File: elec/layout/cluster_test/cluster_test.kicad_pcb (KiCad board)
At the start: 2 copper layers, 31 parts

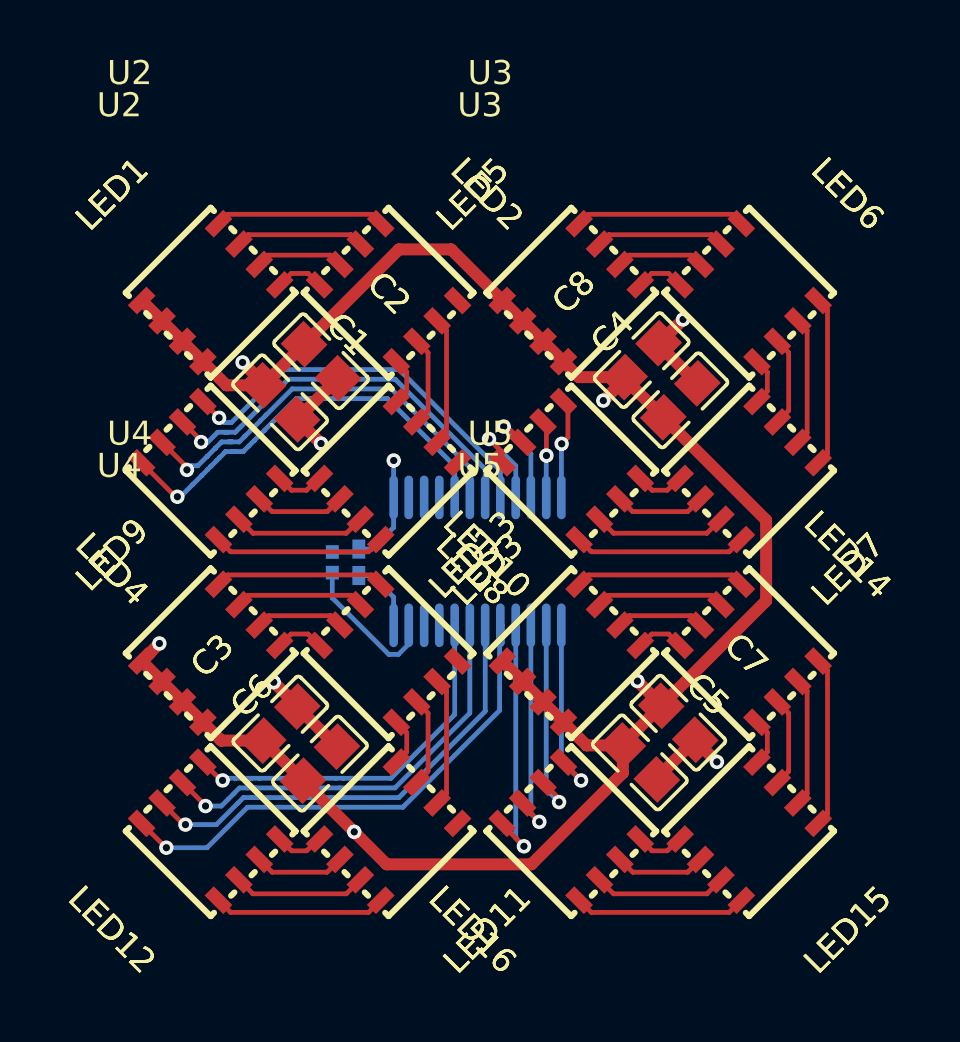
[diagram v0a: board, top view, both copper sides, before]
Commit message: built this
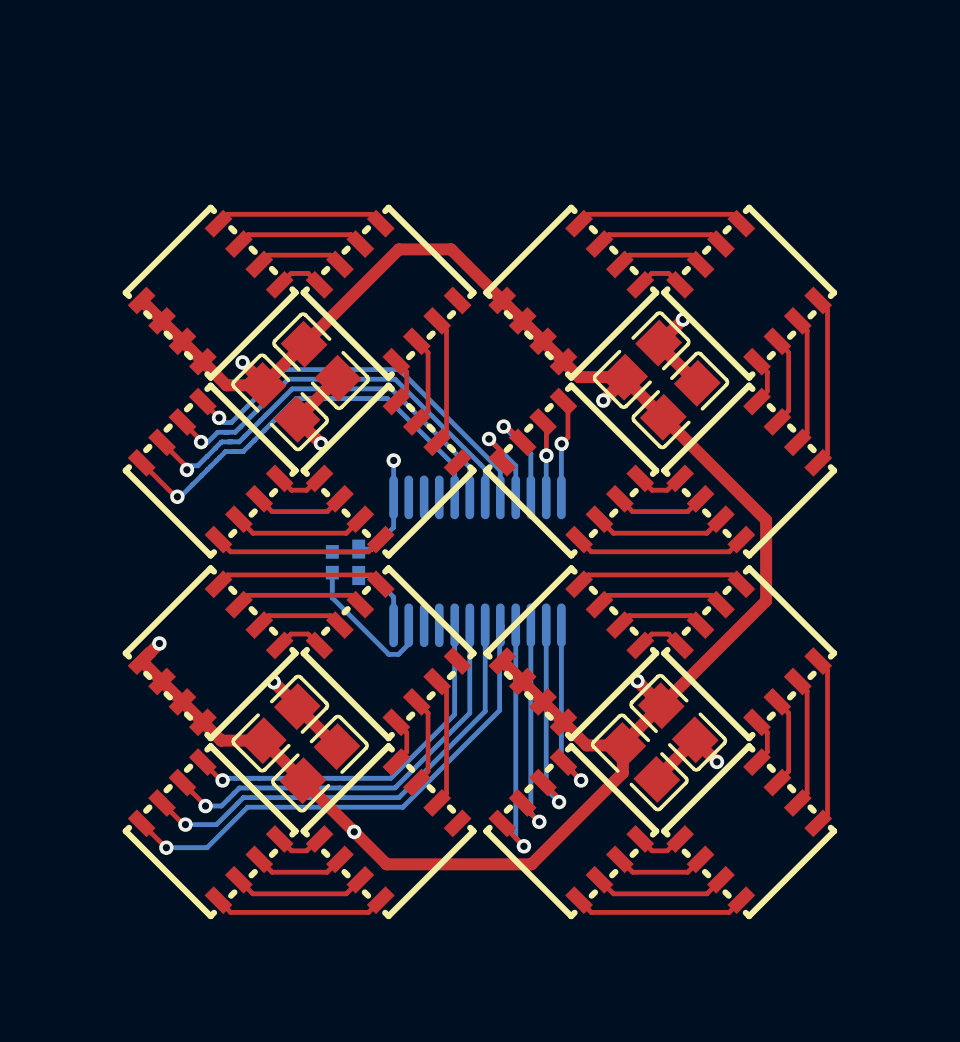
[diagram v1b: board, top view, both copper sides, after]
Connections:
- C1 pad 2: gnd -> cluster-gnd-1
- C2 pad 2: gnd -> cluster-gnd-1
- C3 pad 2: gnd -> cluster-gnd-1
- C4 pad 2: gnd -> cluster-gnd-1
- C5 pad 2: gnd -> cluster-gnd-1
- C6 pad 2: gnd -> cluster-gnd-1
- C7 pad 2: gnd -> cluster-gnd-1
- C8 pad 2: gnd -> cluster-gnd-1
- C9 pad 2: gnd -> cluster-gnd-0
- R1 pad 2: gnd -> cluster-gnd-0
- U1 pad 1: gnd -> cluster-gnd-0
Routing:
- net gnd: track 20.7 -> 0.00 mm, vias 5 -> 0
- net cluster-gnd-1: track 0.00 -> 15.0 mm, vias 0 -> 4
- net cluster-gnd-0: track 0.00 -> 5.76 mm, vias 0 -> 1

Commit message: updating rp2040
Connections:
- net anode renamed power_shim-VCC
- net cluster-blue-0 renamed rgbs[3]-cathodes-cathode-1
- net cluster-blue-1 renamed rgbs[3]-cathodes-cathode-4
- net cluster-blue-2 renamed rgbs[3]-cathodes-cathode-7
- net cluster-blue-3 renamed rgbs[3]-cathodes-cathode-11
- net cluster-cold_white-0 renamed rgbs[3]-cathodes-cathode-0
- net cluster-cold_white-1 renamed rgbs[3]-cathodes-cathode-2
- net cluster-cold_white-2 renamed rgbs[3]-cathodes-cathode-3
- net cluster-cold_white-3 renamed rgbs[3]-cathodes-cathode-10
- net cluster-gnd-0 renamed power-GND
- net cluster-gnd-1 renamed power_shim-GND
- net cluster-green-0 renamed rgbs[3]-cathodes-cathode-5
- net cluster-green-1 renamed rgbs[3]-cathodes-cathode-8
- net cluster-green-2 renamed rgbs[3]-cathodes-cathode-12
- net cluster-green-3 renamed rgbs[3]-cathodes-cathode-15
- net cluster-red-0 renamed rgbs[3]-cathodes-cathode-6
- net cluster-red-1 renamed rgbs[3]-cathodes-cathode-9
- net cluster-red-2 renamed rgbs[3]-cathodes-cathode-13
- net cluster-red-3 renamed rgbs[3]-cathodes-cathode-14
- net cluster.rows[0].pixels[0]-blue-0 renamed rgbs[1]-anodes-anode-0
- net cluster.rows[0].pixels[0]-blue-1 renamed rgbs[2]-anodes-anode-0
- net cluster.rows[0].pixels[0]-blue-2 renamed rgbs[3]-anodes-anode-0
- net cluster.rows[0].pixels[0]-cold_white-0 renamed rgbs[1]-anodes-anode-1
- net cluster.rows[0].pixels[0]-cold_white-1 renamed rgbs[2]-anodes-anode-1
- net cluster.rows[0].pixels[0]-cold_white-2 renamed rgbs[3]-anodes-anode-1
- net cluster.rows[0].pixels[0]-green-0 renamed rgbs[1]-anodes-anode-2
- net cluster.rows[0].pixels[0]-green-1 renamed rgbs[2]-anodes-anode-2
- net cluster.rows[0].pixels[0]-green-2 renamed rgbs[3]-anodes-anode-2
- net cluster.rows[0].pixels[0]-red-0 renamed rgbs[1]-anodes-anode-3
- net cluster.rows[0].pixels[0]-red-1 renamed rgbs[2]-anodes-anode-3
- net cluster.rows[0].pixels[0]-red-2 renamed rgbs[3]-anodes-anode-3
- net cluster.rows[0].pixels[1]-blue-0 renamed rgbs[1]-anodes-anode-4
- net cluster.rows[0].pixels[1]-blue-1 renamed rgbs[2]-anodes-anode-4
- net cluster.rows[0].pixels[1]-blue-2 renamed rgbs[3]-anodes-anode-4
- net cluster.rows[0].pixels[1]-cold_white-0 renamed rgbs[1]-anodes-anode-5
- net cluster.rows[0].pixels[1]-cold_white-1 renamed rgbs[2]-anodes-anode-5
- net cluster.rows[0].pixels[1]-cold_white-2 renamed rgbs[3]-anodes-anode-5
- net cluster.rows[0].pixels[1]-green-0 renamed rgbs[1]-anodes-anode-6
- net cluster.rows[0].pixels[1]-green-1 renamed rgbs[2]-anodes-anode-6
- net cluster.rows[0].pixels[1]-green-2 renamed rgbs[3]-anodes-anode-6
- net cluster.rows[0].pixels[1]-red-0 renamed rgbs[1]-anodes-anode-7
- net cluster.rows[0].pixels[1]-red-1 renamed rgbs[2]-anodes-anode-7
- net cluster.rows[0].pixels[1]-red-2 renamed rgbs[3]-anodes-anode-7
- net cluster.rows[1].pixels[0]-blue-0 renamed rgbs[1]-anodes-anode-8
- net cluster.rows[1].pixels[0]-blue-1 renamed rgbs[2]-anodes-anode-8
- net cluster.rows[1].pixels[0]-blue-2 renamed rgbs[3]-anodes-anode-8
- net cluster.rows[1].pixels[0]-cold_white-0 renamed rgbs[1]-anodes-anode-9
- net cluster.rows[1].pixels[0]-cold_white-1 renamed rgbs[2]-anodes-anode-9
- net cluster.rows[1].pixels[0]-cold_white-2 renamed rgbs[3]-anodes-anode-9
- net cluster.rows[1].pixels[0]-green-0 renamed rgbs[1]-anodes-anode-10
- net cluster.rows[1].pixels[0]-green-1 renamed rgbs[2]-anodes-anode-10
- net cluster.rows[1].pixels[0]-green-2 renamed rgbs[3]-anodes-anode-10
- net cluster.rows[1].pixels[0]-red-0 renamed rgbs[1]-anodes-anode-11
- net cluster.rows[1].pixels[0]-red-1 renamed rgbs[2]-anodes-anode-11
- net cluster.rows[1].pixels[0]-red-2 renamed rgbs[3]-anodes-anode-11
- net cluster.rows[1].pixels[1]-blue-0 renamed rgbs[1]-anodes-anode-12
- net cluster.rows[1].pixels[1]-blue-1 renamed rgbs[2]-anodes-anode-12
- net cluster.rows[1].pixels[1]-blue-2 renamed rgbs[3]-anodes-anode-12
- net cluster.rows[1].pixels[1]-cold_white-0 renamed rgbs[1]-anodes-anode-13
- net cluster.rows[1].pixels[1]-cold_white-1 renamed rgbs[2]-anodes-anode-13
- net cluster.rows[1].pixels[1]-cold_white-2 renamed rgbs[3]-anodes-anode-13
- net cluster.rows[1].pixels[1]-green-0 renamed rgbs[1]-anodes-anode-14
- net cluster.rows[1].pixels[1]-green-1 renamed rgbs[2]-anodes-anode-14
- net cluster.rows[1].pixels[1]-green-2 renamed rgbs[3]-anodes-anode-14
- net cluster.rows[1].pixels[1]-red-0 renamed rgbs[1]-anodes-anode-15
- net cluster.rows[1].pixels[1]-red-1 renamed rgbs[2]-anodes-anode-15
- net cluster.rows[1].pixels[1]-red-2 renamed rgbs[3]-anodes-anode-15
- net hv renamed power-VCC
